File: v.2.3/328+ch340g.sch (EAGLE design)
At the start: 88 parts, among them IC1 LM1117-33, IC2 ENC28J60, K2 G5V1, K3 JRC-21F(4100), T1 2N2222, T2 2N2222, T3 2N2222, T4 2N2222, U1 ATMEGA328P, X1 32.768kHz, X10 22-23-2031, X12 12MHZ, X2 16MHz, X3 25MHz, X9 22-23-2031

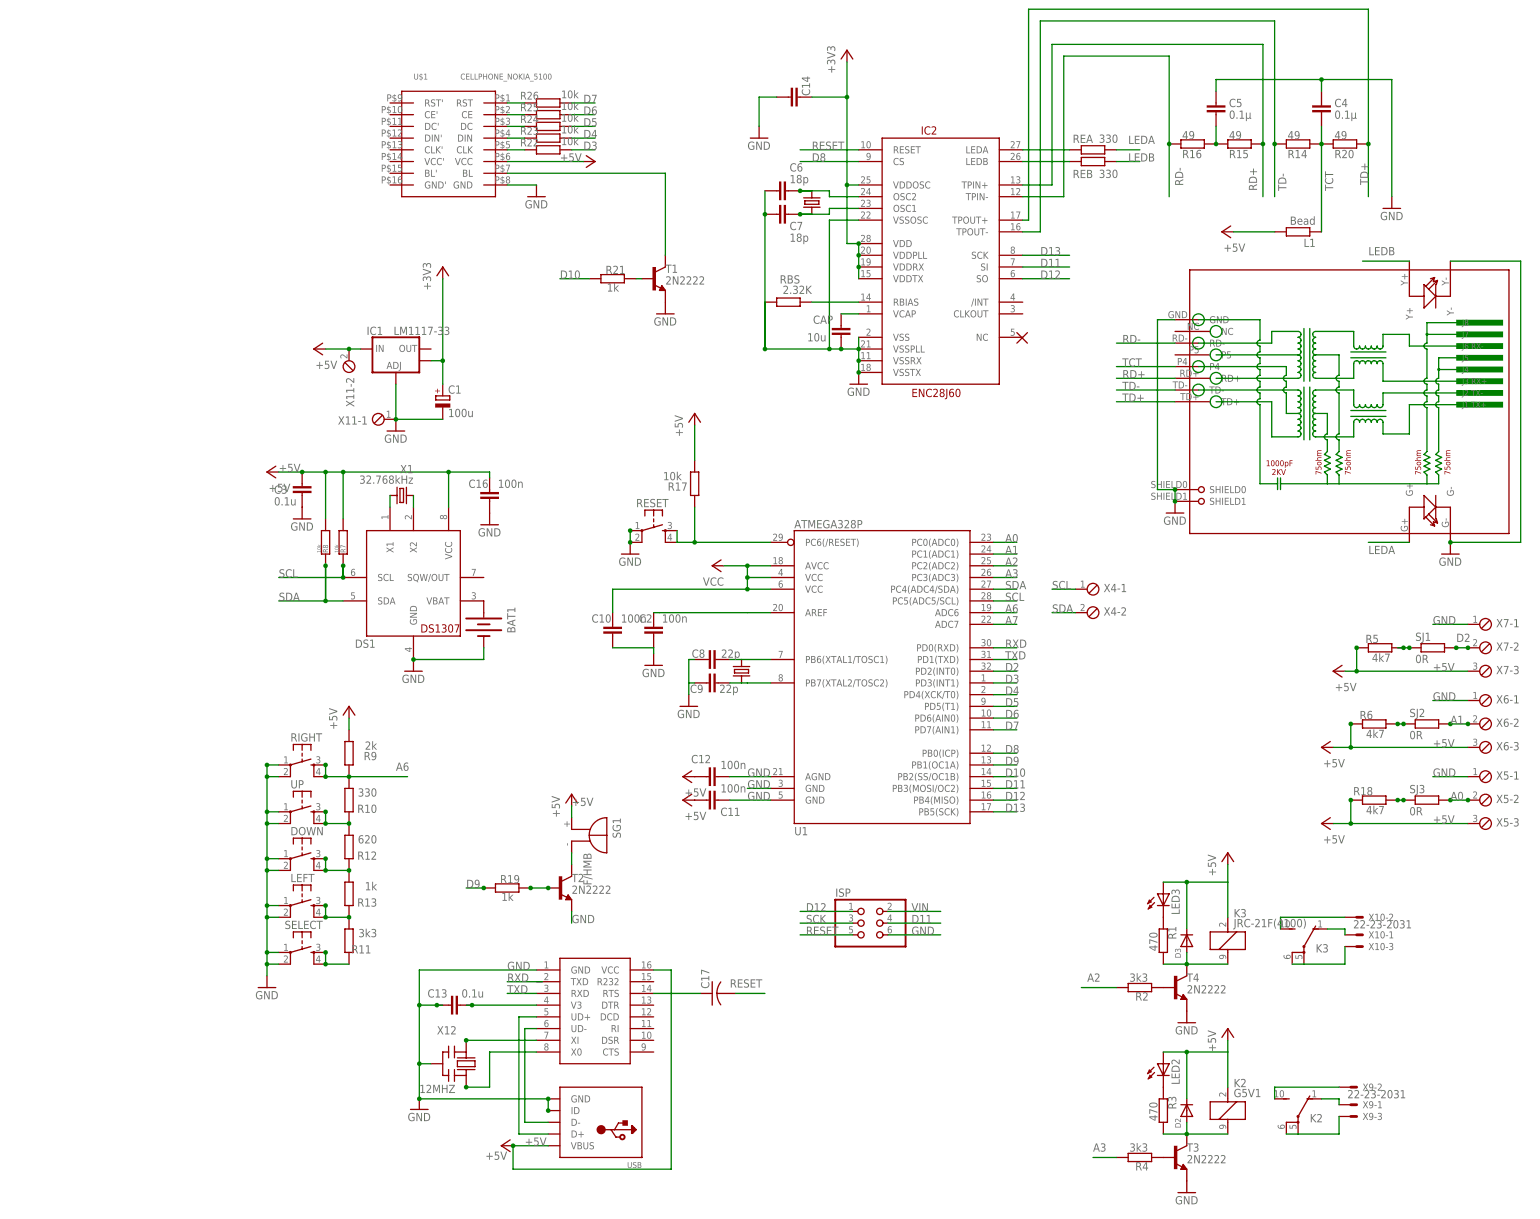
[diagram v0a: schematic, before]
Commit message: 1.3 versija
programa su 3 klavisais
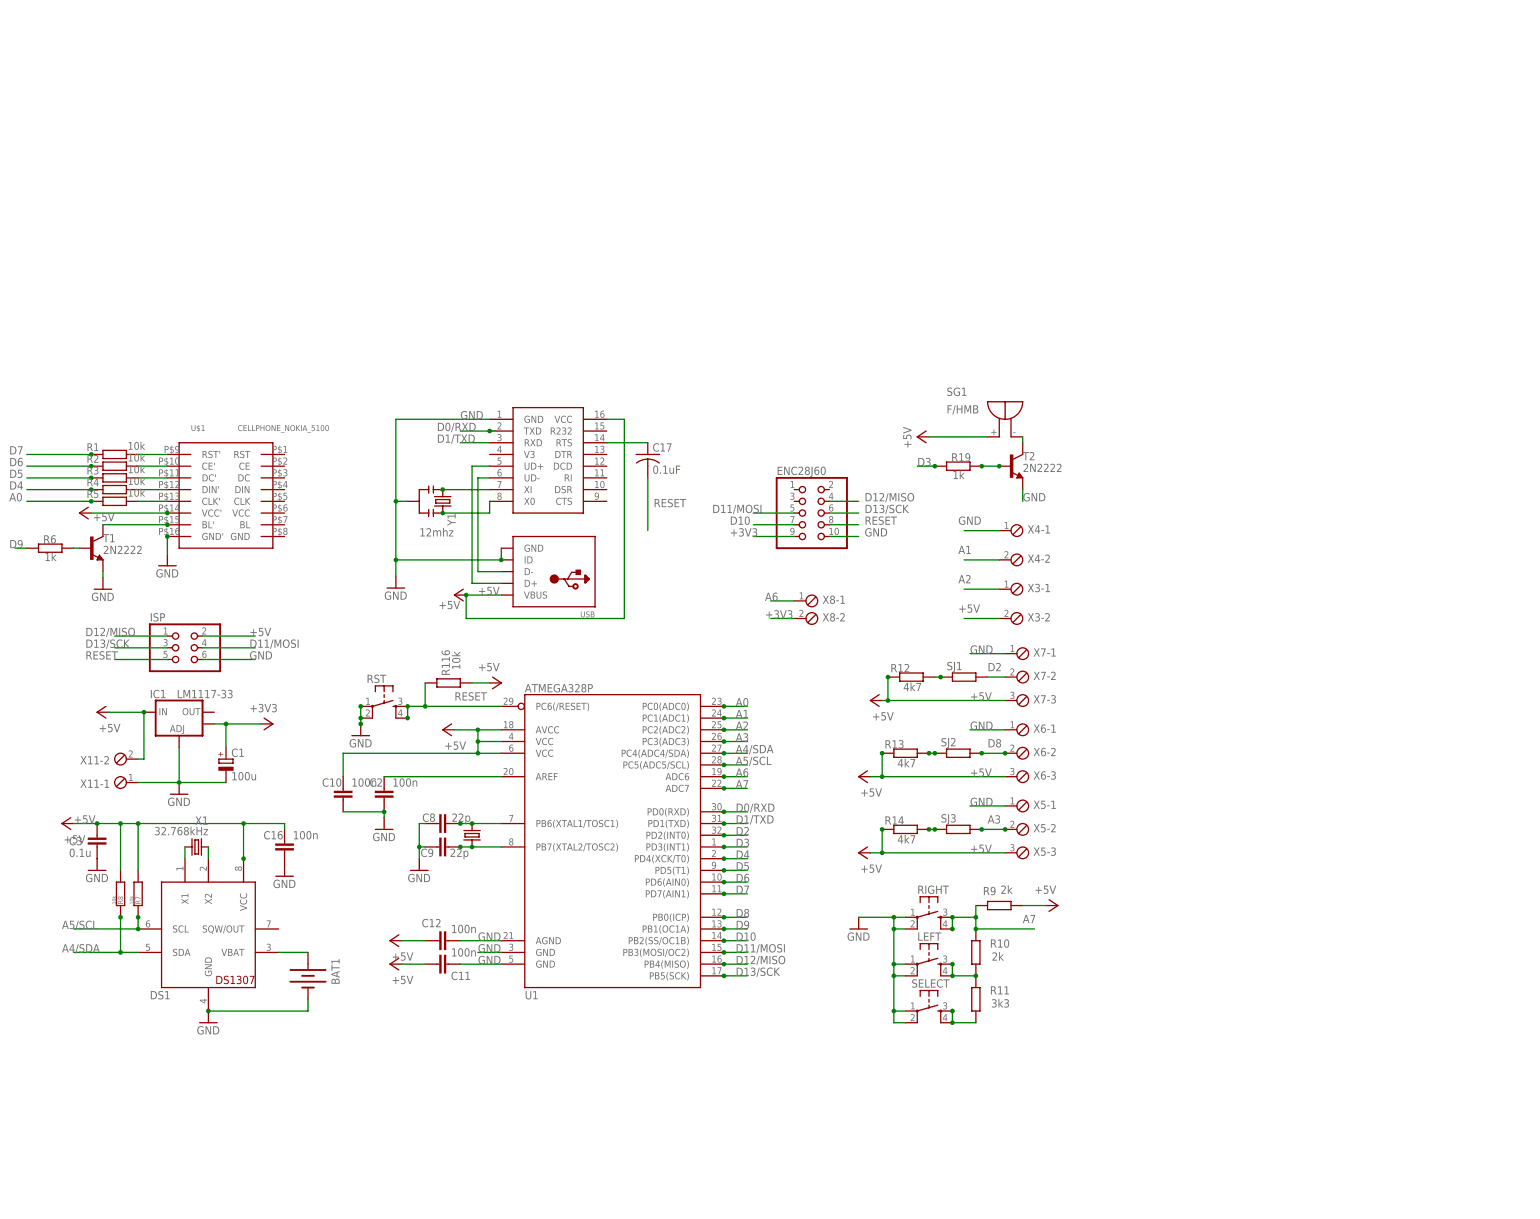
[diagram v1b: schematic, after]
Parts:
- removed C13: 0.1u, rcl:C-EUC0805
- removed C14: 100n, resistor:C-EUC0805
- removed C4, C5: 0.1µ, resistor:C-EUC0805
- removed C6, C7: 18p, resistor:C-EUC0805
- removed CAP: 10u, resistor:C-EUC0805
- removed D2, D3: (no value), adafruit:DIODEDO-1N4148
- removed DOWN, RESET, UP: (no value), SparkFun-Electromechanical:TAC_SWITCHPTH
- removed IC2: ENC28J60, SparkFun-DigitalIC:ENC28J60
- removed K2: G5V1, relay:G5V1
- removed K3: JRC-21F(4100), relay:JRC-21F(4100)
- removed L1: Bead, rcl:R-EU_R0805
- removed LED2, LED3: (no value), adafruit:LEDSMT1206
- removed R15, R16, R20: 49, rcl:R-EU_R0805
- removed R17, R22, R23, R24, R25, R26: 10k, rcl:R-EU_R0805
- removed R18: 4k7, rcl:R-EU_R0805
- removed R21: 1k, rcl:R-EU_R0805
- removed RBS: 2.32K, rcl:R-EU_R0805
- removed REA, REB: 330, rcl:R-EU_R0805
- removed RJ1: HR911105A, CONNECTER:HR911105A
- removed T3, T4: 2N2222, adafruit:2N2222
- removed X10, X9: 22-23-2031, con-molex:22-23-2031
- removed X12: 12MHZ, adafruit:CERMOSCILL-THM
- added ENC28J60: (no value), pinhead:PINHD-2X5
- added R116: 10k, rcl:R-EU_R0805
- added RST: (no value), SparkFun-Electromechanical:TAC_SWITCHPTH
- added X8: (no value), con-phoenix-254:MPT2
- added Y1: 12mhz, SparkFun-FreqCtrl:RESONATORPTH
- BAT1, ISP, LEFT, RIGHT, SELECT, USB, X11, X5, X6, X7: value (none) -> (none)
- C17: value (none) -> 0.1uF
- R1, R3: value 470 -> 10k
- R10: value 330 -> 2k
- R12: value 620 -> 4k7
- R13: value 1k -> 4k7
- R14: value 49 -> 4k7
- R2, R4: value 3k3 -> 10k
- R5: value 4k7 -> 10k
- R6: value 4k7 -> 1k
- SJ1, SJ2, SJ3: value 0R -> (none)
- X3: value 25MHz -> (none); device SparkFun:CRYSTALHC49US -> con-phoenix-254:MPT2
- X4: value (none) -> (none); OC_FARNELL unknown -> (none); OC_NEWARK unknown -> (none)
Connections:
- net TXD renamed D1/TXD
- removed net D11: IC2.SI, ISP.4, U1.PB3(MOSI/OC2)
- removed net D12: IC2.SO, ISP.1, U1.PB4(MISO)
- removed net D13: IC2.SCK, U1.PB5(SCK)
- removed net LEDA: REA.2, RJ1.G+
- removed net LEDB: REB.2, RJ1.Y+
- removed net N$12: D3.A, K31.2, R1.2, T4.C
- removed net N$13: R2.1, T4.B
- removed net N$14: K22.O, X9-1.S
- removed net N$16: K32.S, X10-2.S
- removed net N$19: K32.P, K32.P@1, X10-3.S
- removed net N$20: K32.O, X10-1.S
- removed net N$21: LED3.C, R1.1
- removed net N$22: R22.1, U$1.CLK
- removed net N$23: R25.1, U$1.CE
- removed net N$24: R24.1, U$1.DC
- removed net N$25: R23.1, U$1.DIN
- removed net N$34: IC2.LEDA, REA.1
- removed net N$37: IC2.LEDB, REB.1
- removed net N$38: U$2.X0, X12.OUT
- removed net N$39: CAP.1, IC2.VCAP
- removed net N$41: C6.1, IC2.OSC2, X3.2
- removed net N$42: C7.1, IC2.OSC1, X3.1
- removed net N$46: R17.1, RESET.3, RESET.4, U1.PC6(/RESET)
- removed net N$54: C5.2, R15.1, R16.2
- removed net N$59: IC2.RBIAS, RBS.2
- removed net N$7 (its old number): LED2.C, R3.1
- removed net N$9: R10.1, R12.2, UP.3, UP.4
- removed net RD+: IC2.TPIN+, R15.2, RJ1.RD+
- removed net RD-: IC2.TPIN-, R16.1, RJ1.RD-
- removed net RXD: U1.PD0(RXD)
- removed net SCK: ISP.3
- removed net SCL: DS1.SCL, R7.1, U1.PC5(ADC5/SCL), X4-1.1
- removed net SDA: DS1.SDA, R8.1, U1.PC4(ADC4/SDA), X4-2.1
- removed net TCT: C4.2, L1.1, R14.2, R20.1, RJ1.P4
- removed net TD+: IC2.TPOUT+, R20.2, RJ1.TD+
- removed net TD-: IC2.TPOUT-, R14.1, RJ1.TD-
- removed net V$: R26.1, U$1.RST
- removed net VIN: ISP.2
- new net A4/SDA: DS1.SDA, R8.1, U1.PC4(ADC4/SDA)
- new net A5/SCL: DS1.SCL, R7.1, U1.PC5(ADC5/SCL)
- new net D0/RXD: U$2.TXD, U1.PD0(RXD)
- new net D11/MOSI: ENC28J60.5, ISP.4, U1.PB3(MOSI/OC2)
- new net D12/MISO: ENC28J60.4, ISP.1, U1.PB4(MISO)
- new net D13/SCK: ENC28J60.6, ISP.3, U1.PB5(SCK)
- net +3V3: now also ENC28J60.9, X8-2.1; no longer C14.1, IC2.VDD, IC2.VDDOSC, IC2.VDDPLL, IC2.VDDRX, IC2.VDDTX
- net +5V: now also ISP.2, R116.2, R12.1, R13.1, R14.1, U$1.VCC', X3-2.1; no longer D2.C, D3.C, K21.1, K31.1, L1.2, LED2.A, LED3.A, R17.2, R18.1, R5.1, R6.1, U$1.VCC
- net A0: now also R5.1; no longer SJ3.2, X5-2.1
- net A1: now also X4-2.1; no longer SJ2.2, X6-2.1
- net A2: now also X3-1.1; no longer R2.2
- net A3: now also SJ3.2, X5-2.1; no longer R4.2
- net A6: now also X8-1.1; no longer R10.2, R9.1, RIGHT.3, RIGHT.4
- net A7: now also R10.2, R9.1, RIGHT.3, RIGHT.4
- net D10: now also ENC28J60.7; no longer R21.2
- net D3: now also R19.2; no longer R22.2
- net D4: now also R4.1; no longer R23.2
- net D5: now also R3.1; no longer R24.2
- net D6: now also R2.1; no longer R25.2
- net D7: now also R1.1; no longer R26.2
- net D8: now also SJ2.2, X6-2.1; no longer IC2.CS
- net D9: now also R6.2; no longer R19.2
- net GND: now also ENC28J60.10, RST.1, RST.2, U$1.GND', X4-1.1, Y1.2; no longer C13.1, C14.2, C4.1, C5.1, C6.2, C7.2, CAP.2, DOWN.1, DOWN.2, IC2.VSS, IC2.VSSOSC, IC2.VSSPLL, IC2.VSSRX, IC2.VSSTX, RBS.1, RESET.1, RESET.2, RJ1.G-, RJ1.GND, RJ1.SHIELD0, RJ1.SHIELD1, RJ1.Y-, T3.E, T4.E, U$1.GND, UP.1, UP.2, X12.GND
- net N$1: now also R10.1; no longer R13.1
- net N$10: now also Y1.1; no longer X12.IN
- net N$17: now also R13.2; no longer R6.2
- net N$2: now also R5.2, U$1.CLK'; no longer D2.A, K21.2, R3.2, T3.C
- net N$26: now also U$1.BL'; no longer U$1.BL
- net N$28: now also R14.2; no longer R18.2
- net N$3: now also R4.2, U$1.DIN'; no longer R4.1, T3.B
- net N$31: now also R12.2; no longer R5.2
- net N$4: now also R3.2, U$1.DC'; no longer K22.P, K22.P@1, X9-3.S
- net N$40: now also U$2.X0, Y1.3; no longer C13.2, U$2.V3
- net N$44: now also R6.1; no longer R21.1
- net N$5: now also R2.2, U$1.CE'; no longer K22.S, X9-2.S
- net N$6: now also R1.2, U$1.RST'; no longer DOWN.3, DOWN.4, R12.1, R13.2
- net RESET: now also ENC28J60.8, R116.1, RST.3, RST.4, U1.PC6(/RESET); no longer IC2.RESET
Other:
- moved on the sheet: BAT1, C1, C10, C11, C12, C16, C17, C2, C3, C8, C9, DS1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
